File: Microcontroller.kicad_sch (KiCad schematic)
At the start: 1 part, among them U1 ATmega328-A

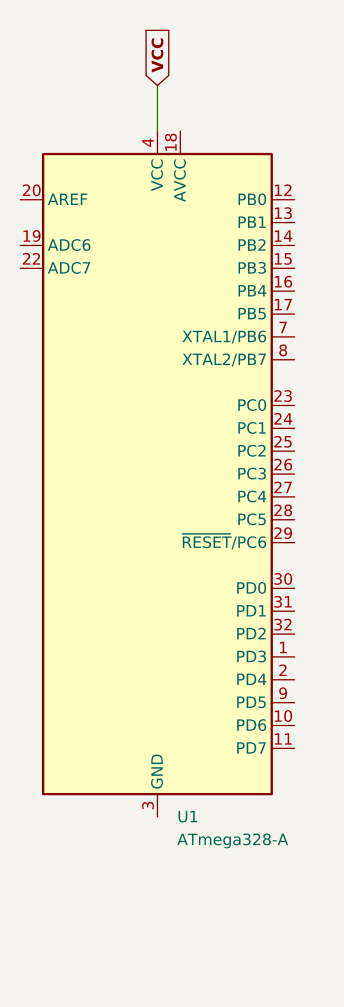
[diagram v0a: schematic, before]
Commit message: Atmega34u4
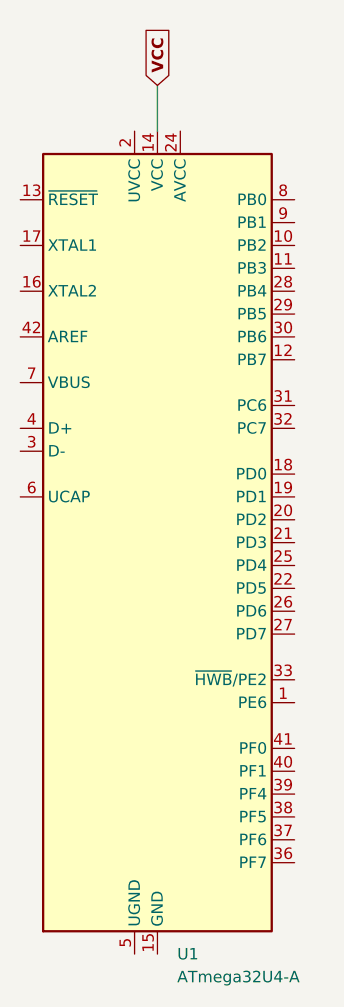
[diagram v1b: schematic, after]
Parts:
- removed U1: ATmega328-A, Package_QFP:TQFP-32_7x7mm_P0.8mm, symbol MCU_Microchip_ATmega:ATmega328-A
- added U1: ATmega32U4-A, Package_QFP:TQFP-44_10x10mm_P0.8mm, symbol MCU_Microchip_ATmega:ATmega32U4-A
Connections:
- net VCC: now also U1.14 (VCC), U1.34 (VCC)
- new net: U1.15 (GND), U1.23 (GND), U1.35 (GND), U1.43 (GND)
- new net: U1.24 (AVCC), U1.44 (AVCC)
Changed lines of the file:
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@@
 	)
 	(symbol
-		(lib_id "MCU_Microchip_ATmega:ATmega328-A")
-		(at 100.33 105.41 0)
+		(lib_id "MCU_Microchip_ATmega:ATmega32U4-A")
+		(at 100.33 113.03 0)
 		(unit 1)
 		(exclude_from_sim no)
@@
 		(fields_autoplaced yes)
 		(property "Reference" "U1"
-			(at 102.5241 143.51 0)
+			(at 102.5241 158.75 0)
 			(effects
 				(font
@@
 			)
 		)
-		(property "Value" "ATmega328-A"
-			(at 102.5241 146.05 0)
+		(property "Value" "ATmega32U4-A"
+			(at 102.5241 161.29 0)
 			(effects
 				(font
@@
 			)
 		)
-		(property "Footprint" "Package_QFP:TQFP-32_7x7mm_P0.8mm"
-			(at 100.33 105.41 0)
+		(property "Footprint" "Package_QFP:TQFP-44_10x10mm_P0.8mm"
+			(at 100.33 113.03 0)
 			(effects
 				(font
@@
 			)
 		)
-		(property "Datasheet" "http://ww1.microchip.com/downloads/en/DeviceDoc/ATmega328_P%20AVR%20MCU%20with%20picoPower%20Technology%20Data%20Sheet%2040001984A.pdf"
-			(at 100.33 105.41 0)
+		(property "Datasheet" "http://ww1.microchip.com/downloads/en/DeviceDoc/Atmel-7766-8-bit-AVR-ATmega16U4-32U4_Datasheet.pdf"
+			(at 100.33 113.03 0)
 			(effects
 				(font
@@
 			)
 		)
-		(property "Description" "20MHz, 32kB Flash, 2kB SRAM, 1kB EEPROM, TQFP-32"
-			(at 100.33 105.41 0)
+		(property "Description" "16MHz, 32kB Flash, 2.5kB SRAM, 1kB EEPROM, USB 2.0, TQFP-44"
+			(at 100.33 113.03 0)
 			(effects
 				(font
@@
 			)
 		)
+		(pin "28"
+		)
+		(pin "42"
+		)
+		(pin "31"
+		)
 		(pin "32"
+		)
+		(pin "36"
+		)
+		(pin "41"
+		)
+		(pin "10"
+		)
+		(pin "33"
+		)
+		(pin "30"
+		)
+		(pin "2"
+		)
+		(pin "38"
+		)
+		(pin "40"
+		)
+		(pin "5"
+		)
+		(pin "6"
+		)
+		(pin "20"
+		)
+		(pin "44"
+		)
+		(pin "7"
+		)
+		(pin "22"
+		)
+		(pin "37"
+		)
+		(pin "23"
+		)
+		(pin "24"
+		)
+		(pin "35"
+		)
+		(pin "26"
+		)
+		(pin "34"
+		)
+		(pin "4"
+		)
+		(pin "12"
+		)
+		(pin "43"
 		)
 		(pin "9"
 		)
+		(pin "13"
+		)
+		(pin "29"
+		)
+		(pin "39"
+		)
+		(pin "21"
+		)
+		(pin "25"
+		)
+		(pin "17"
+		)
+		(pin "18"
+		)
 		(pin "15"
-		)
-		(pin "20"
-		)
-		(pin "6"
 		)
 		(pin "19"
 		)
-		(pin "30"
+		(pin "1"
 		)
-		(pin "4"
+		(pin "11"
 		)
-		(pin "5"
+		(pin "3"
+		)
+		(pin "27"
+		)
+		(pin "8"
+		)
+		(pin "14"
 		)
 		(pin "16"
 		)
-		(pin "18"
-		)
-		(pin "24"
-		)
-		(pin "11"
-		)
-		(pin "12"
-		)
-		(pin "10"
-		)
-		(pin "21"
-		)
-		(pin "14"
-		)
-		(pin "13"
-		)
-		(pin "23"
-		)
-		(pin "2"
-		)
-		(pin "7"
-		)
-		(pin "31"
-		)
-		(pin "1"
-		)
-		(pin "27"
-		)
-		(pin "17"
-		)
-		(pin "3"
-		)
-		(pin "22"
-		)
-		(pin "25"
-		)
-		(pin "28"
-		)
-		(pin "8"
-		)
-		(pin "29"
-		)
-		(pin "26"
-		)
 		(instances
-			(project "EEProject"
+			(project ""
 				(path "/3aa1ef99-b297-42d2-a07b-7cd664ecf53c/681e2464-01d4-4174-9887-b09f82d30530"
 					(reference "U1")
